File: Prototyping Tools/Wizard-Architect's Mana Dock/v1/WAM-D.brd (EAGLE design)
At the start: 104 x 132.7 mm, 0 parts

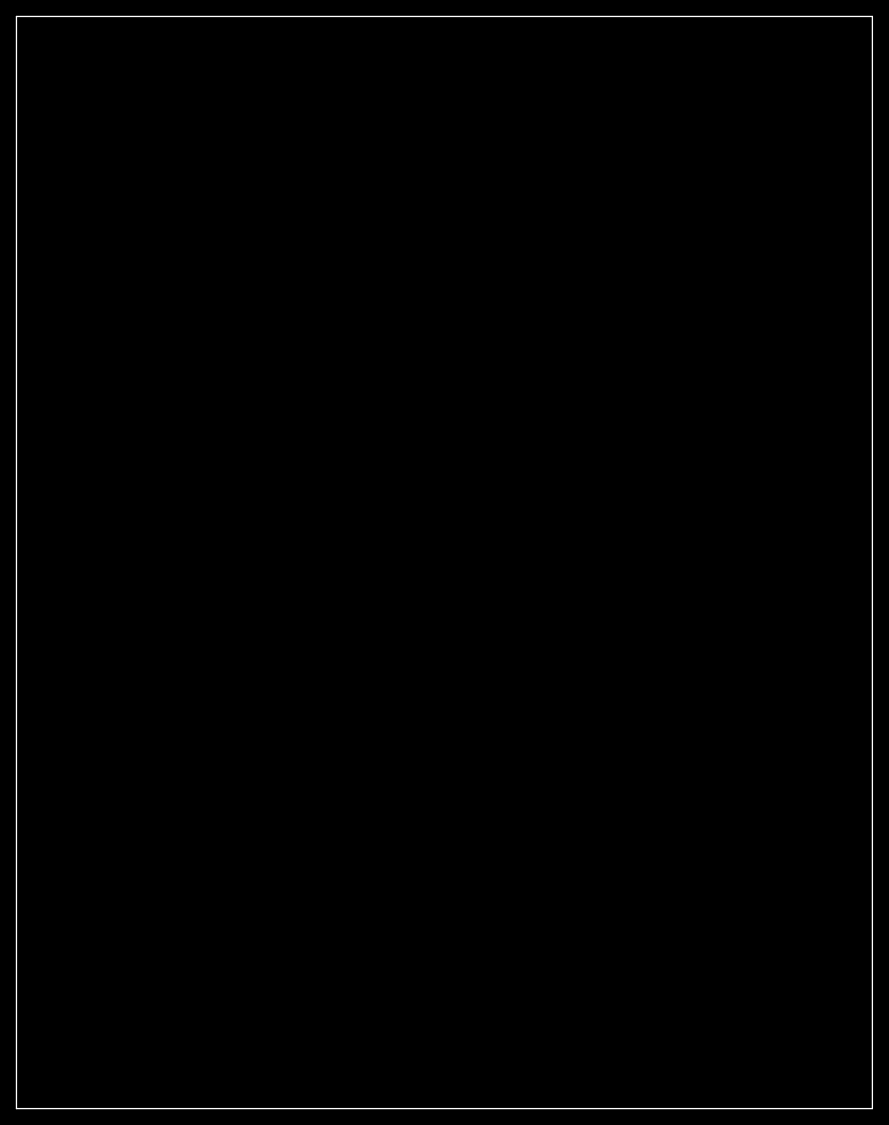
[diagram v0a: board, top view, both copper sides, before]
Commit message: WAM-D progress
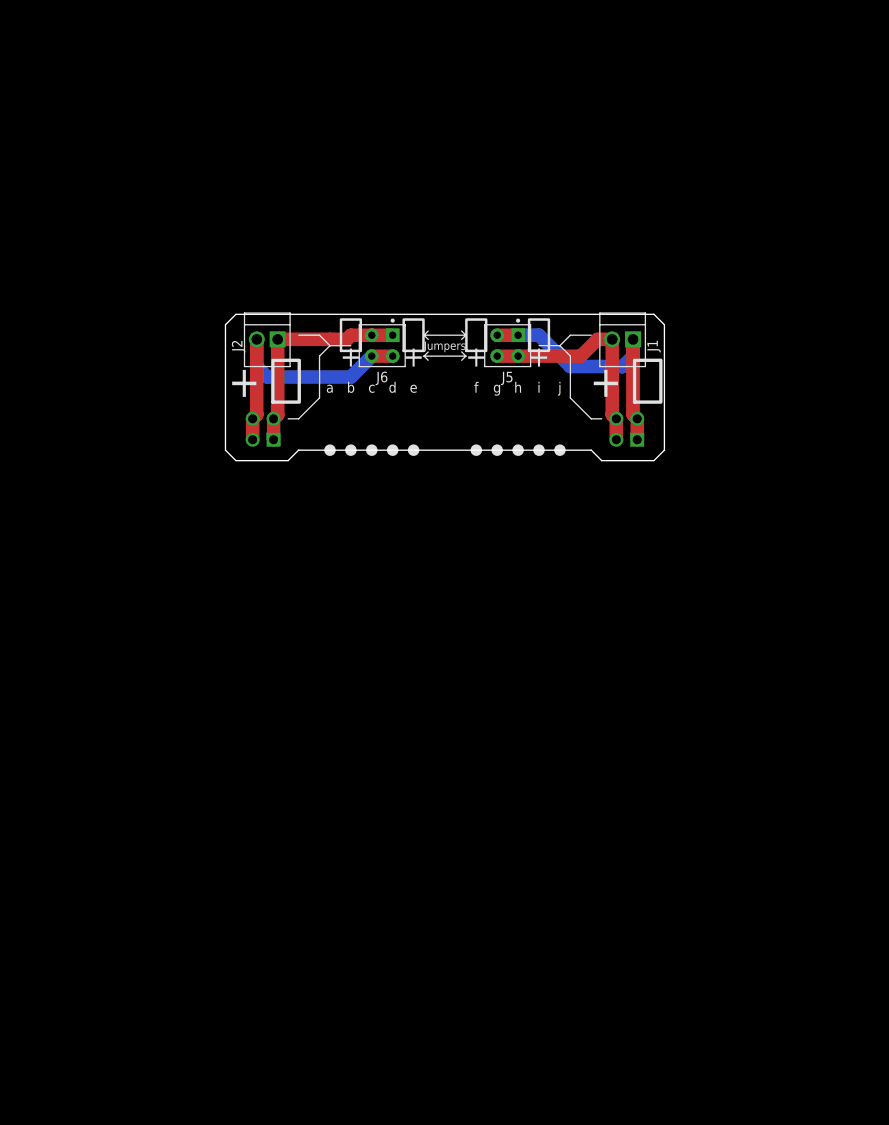
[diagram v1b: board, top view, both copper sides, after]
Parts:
- added J1, J2: OSTVN02A150, SonicAthame:OSTVN02A150
- added J3, J4: M20-9760246, SonicAthame:HDRV4W64P254_2X2_508X508X834B
- added J5, J6: HEADER-2X2-F-8.5, SonicAthame:HDRVR4W75P254_2X2_558X508X850B
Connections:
- new net N$5: J2.P$1, J4.1, J4.2, J6.1, J6.2
- new net N$6: J2.P$2, J4.3, J4.4, J6.3, J6.4
- new net N$7: J1.P$2, J3.3, J3.4, J5.3, J5.4
- new net N$8: J1.P$1, J3.1, J3.2, J5.1, J5.2
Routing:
- net N$6: track 0.00 -> 33.8 mm
- net N$8: track 0.00 -> 33.0 mm
- net N$7: track 0.00 -> 27.2 mm
- net N$5: track 0.00 -> 26.6 mm
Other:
- board size 104 x 132.7 mm -> 53.3 x 17.8 mm
- board text added: "Jumpers"
